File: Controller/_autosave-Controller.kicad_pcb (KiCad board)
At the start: 2 copper layers, 50 parts, among them J1 AudioJack3_SwitchTR, J16 EXT MODULE, J17 EXT MODULE, J3 EURO_CONN, J4 AudioJack3_SwitchTR, J5 AudioJack3_SwitchTR, J6 AudioJack3_SwitchTR, J7 AudioJack3_SwitchTR, U1 TL074, U2 TL074

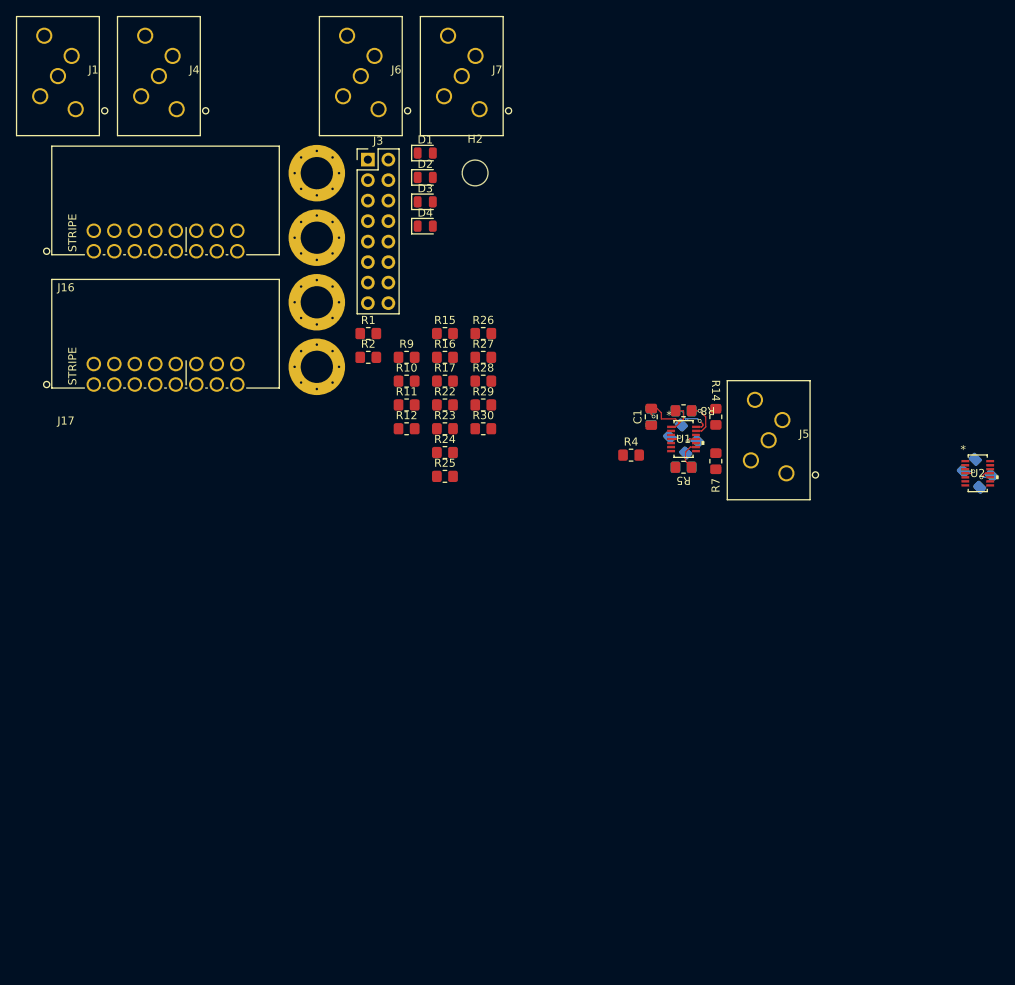
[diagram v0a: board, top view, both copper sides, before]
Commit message: GET IT ON GITHUB NAO!
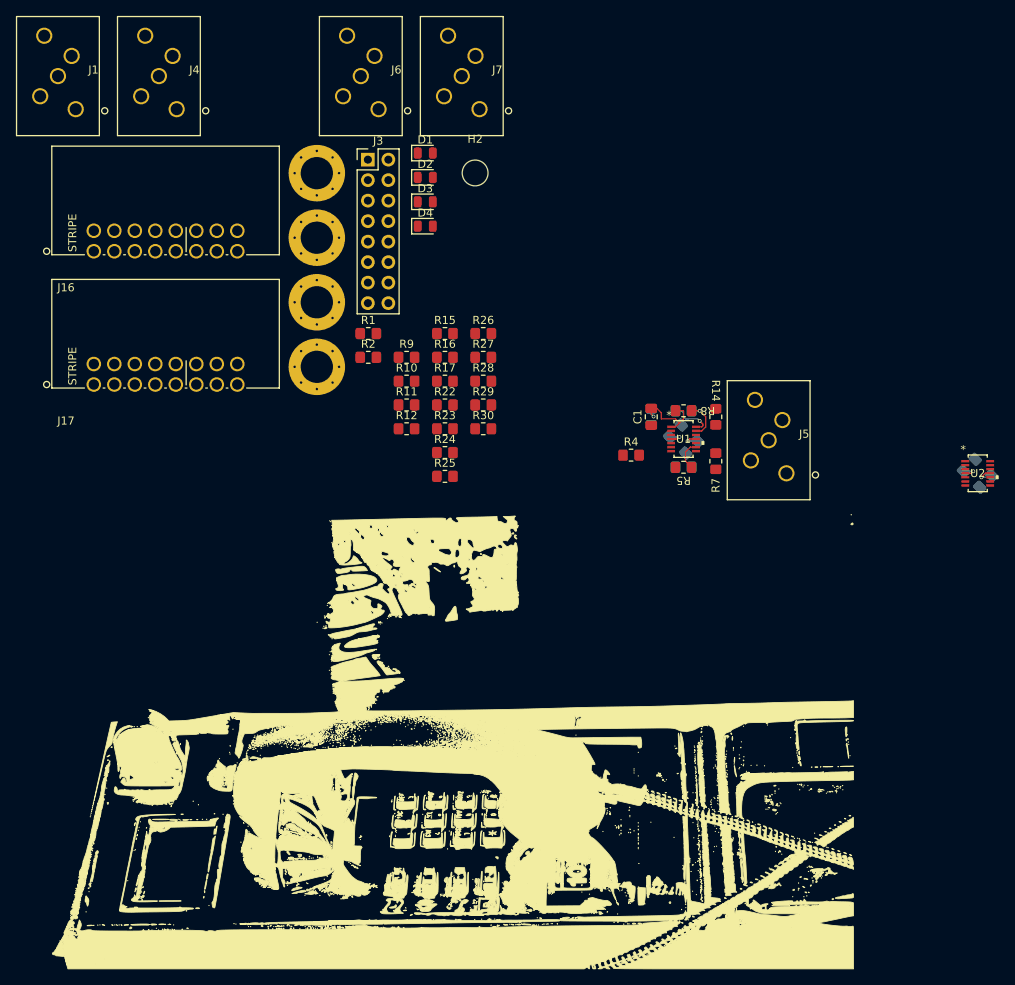
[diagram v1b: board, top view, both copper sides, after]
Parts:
- added G***: LOGO, AT-Footprints:gfx_ehlo_backgr, F.Cu at (117.8, 134.9)
